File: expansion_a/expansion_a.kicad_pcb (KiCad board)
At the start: 4 copper layers, 60.5 x 56 mm, 50 parts, among them J101 Conn_01x08, J1101 Conn_01x03, J1102 Conn_01x06, J201 Conn_01x03, J202 Conn_01x06, U1001 GAQY212G1S, U101 74HC373, U102 74HC595, U301 GAQY212G1S, U401 GAQY212G1S, U501 GAQY212G1S, U601 GAQY212G1S, U701 GAQY212G1S, U801 GAQY212G1S, U901 GAQY212G1S

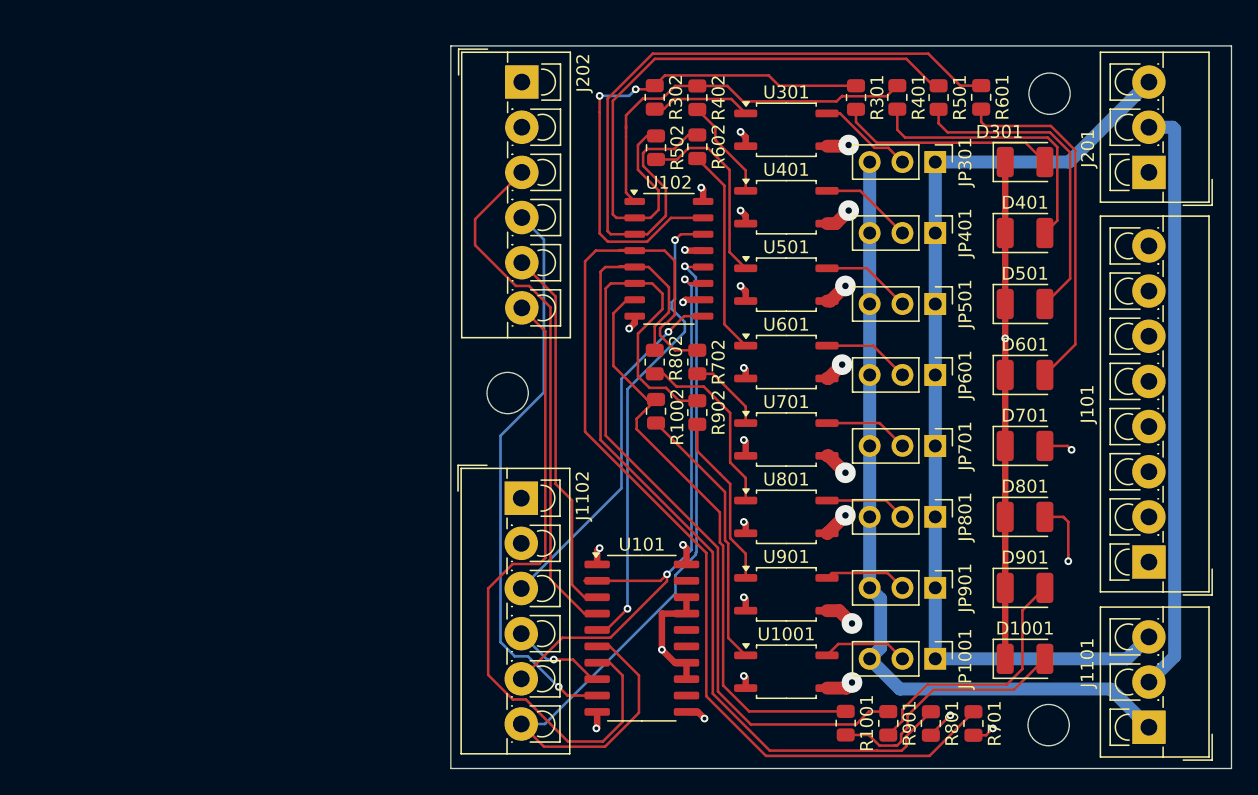
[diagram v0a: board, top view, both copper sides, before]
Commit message: Finalise expansion A.
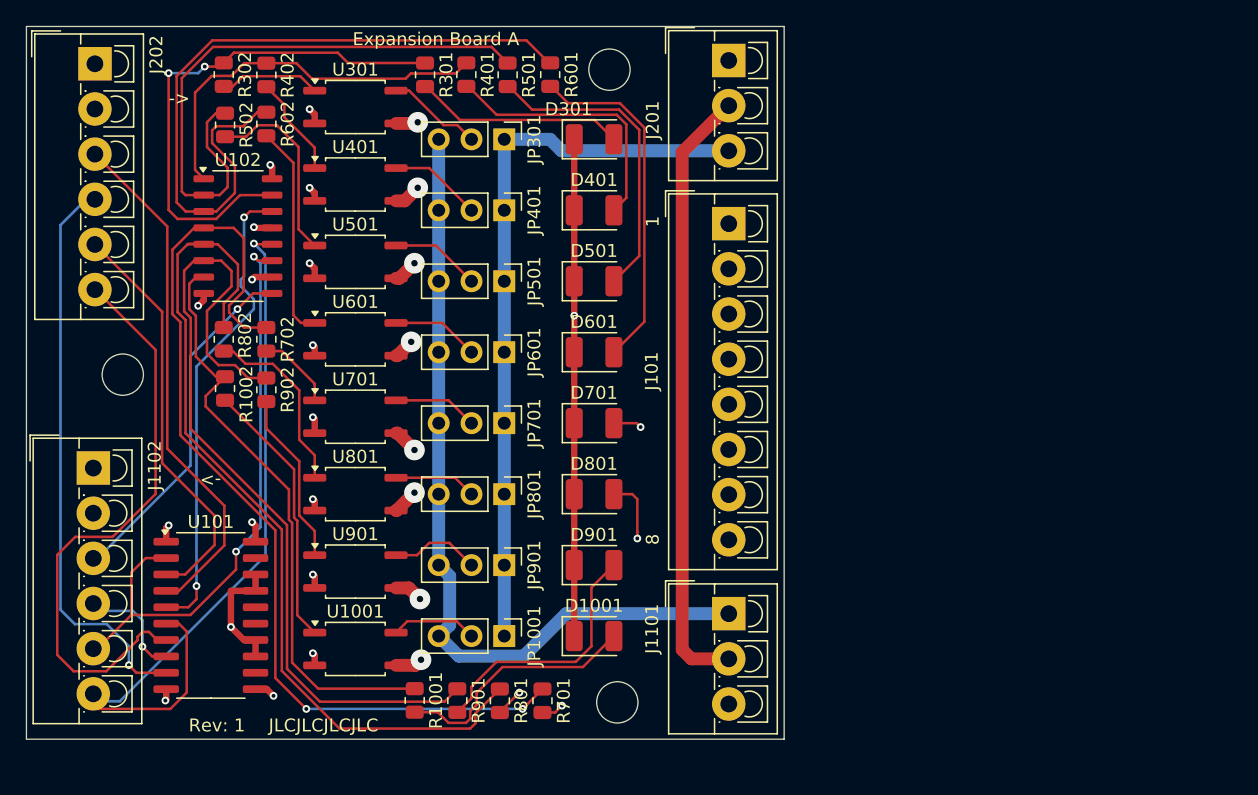
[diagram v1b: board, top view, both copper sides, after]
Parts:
- moved J101 41.8 mm to (123.0, 49.3), turned to -90 degrees
- moved REF2 34.2 mm to (113.8, 37.3)
- moved J1101 33.7 mm to (123.0, 79.5), turned to -90 degrees
- moved J201 33.7 mm to (123.0, 36.6), turned to -90 degrees
- moved REF3 33.5 mm to (114.4, 86.4)
- moved R1002 33.4 mm to (84.0, 62.0)
- moved R301 33.4 mm to (99.5, 37.7)
- moved R501 33.4 mm to (105.9, 37.7)
- moved R502 33.4 mm to (84.0, 41.6)
- moved R901 33.4 mm to (102.0, 86.2)
- moved U102 33.4 mm to (85.0, 50.2)
- moved D1001 33.4 mm to (112.6, 81.2)
- moved D301 33.4 mm to (112.6, 42.7)
- moved D401 33.4 mm to (112.6, 48.2)
- moved D501 33.4 mm to (112.6, 53.7)
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- renumbered REF** to REF1, REF** to REF2, REF** to REF3
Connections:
- J101 pad 1: /out8 -> /out1
- J101 pad 2: /out7 -> /out2
- J101 pad 3: /out6 -> /out3
- J101 pad 4: /out5 -> /out4
- J101 pad 5: /out4 -> /out5
- J101 pad 6: /out3 -> /out6
- J101 pad 7: /out2 -> /out7
- J101 pad 8: /out1 -> /out8
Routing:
- net /Connector in/CS: track 51.4 -> 45.5 mm
- net /set5: track 80.2 -> 75.0 mm, vias 0 -> 2
- net /Connector out/CS: track 62.0 -> 59.1 mm
- net /Connector in/CLK: track 28.9 -> 31.8 mm
- net Vdrive: track 86.3 -> 88.7 mm
- net GNDPWR: track 45.7 -> 47.6 mm
- net /set7: track 67.1 -> 65.7 mm
- net /Connector out/MISO: track 7.34 -> 8.53 mm
- net /set6: track 69.0 -> 67.9 mm
- net VSS: track 74.9 -> 75.8 mm
- net Net-(D401-A): track 21.6 -> 20.7 mm
- net /set4: track 57.3 -> 56.4 mm
- net /out5: track 27.0 -> 27.8 mm
- net /out8: track 30.7 -> 31.5 mm
- net /set1: track 41.5 -> 40.7 mm
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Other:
- board size 60.5 x 56 mm -> 58.7 x 55.2 mm
- board text added: "->"
- board text added: "1"
- board text added: "8"
- board text added: "Expansion Board A"
- board text added: "JLCJLCJLCJLC"
- board text added: "Rev: 1"
